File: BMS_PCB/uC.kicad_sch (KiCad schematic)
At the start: 2 parts, among them J2 Conn_01x09, U7 STM32F407G-DISC1

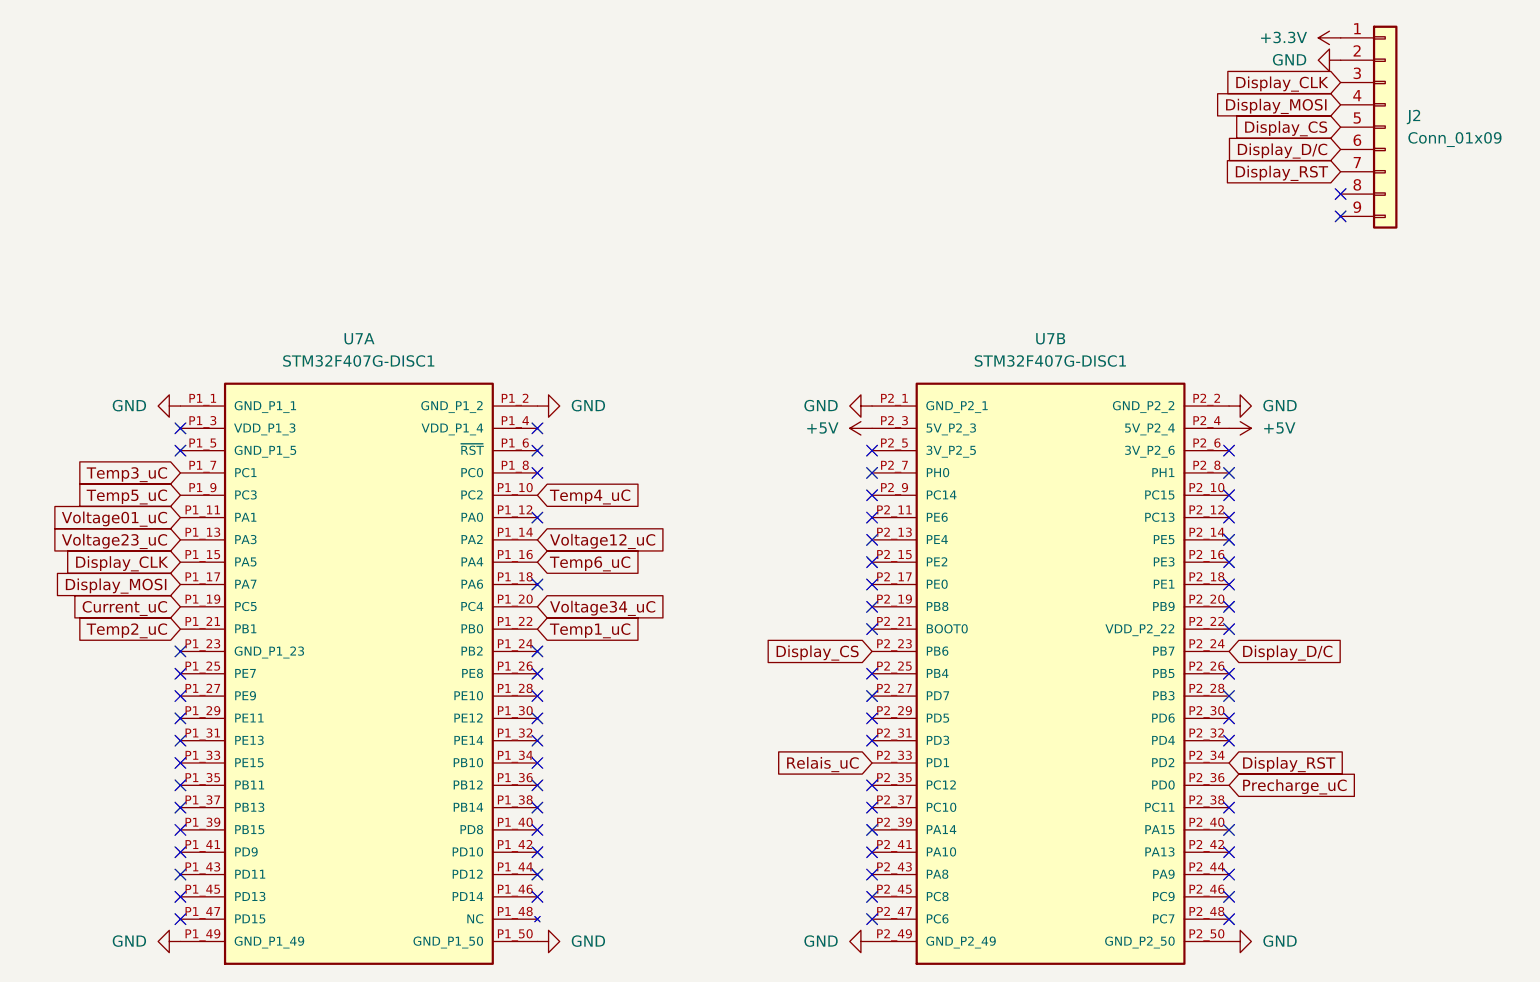
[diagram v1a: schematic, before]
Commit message: Footprints changes
-U10
-uC pins/SPI changes
- Fuses
- DSUB
- reupload layout
- etc.
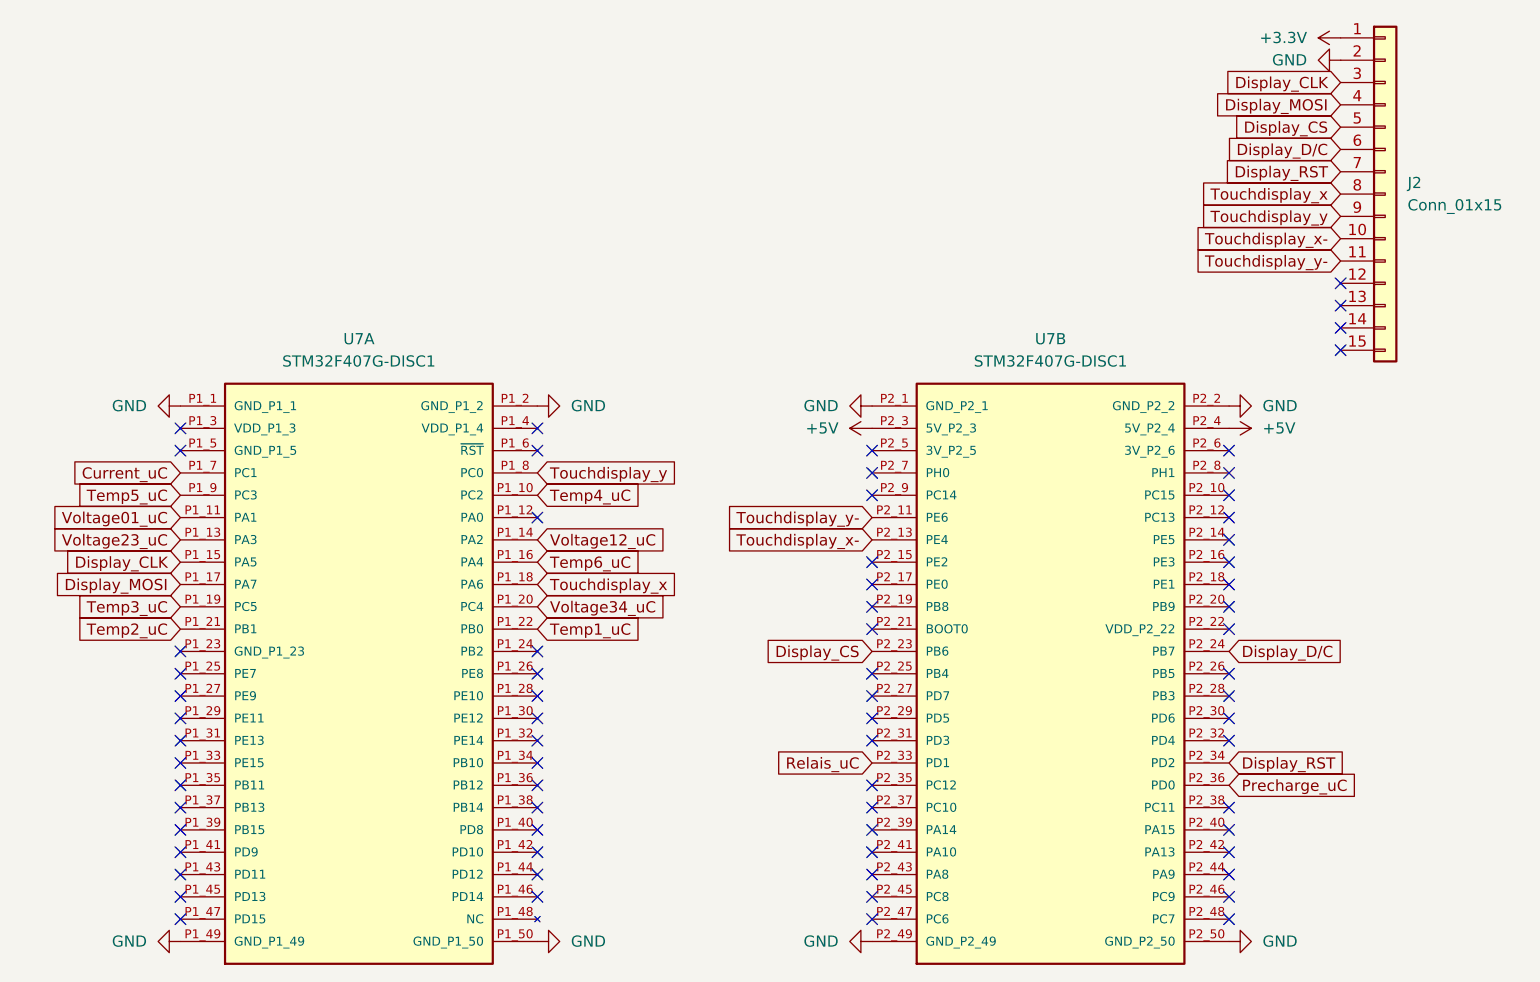
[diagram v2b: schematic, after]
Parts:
- removed J2: Conn_01x09, Connector_Dsub:DSUB-9_Socket_Horizontal_P2.77x2.84mm_EdgePinOffset14.56mm_Housed_MountingHolesOffset15.98mm, symbol Connector_Generic:Conn_01x09
- added J2: Conn_01x15, Connector_Dsub:DSUB-15_Socket_Horizontal_P2.77x2.84mm_EdgePinOffset14.56mm_Housed_MountingHolesOffset15.98mm, symbol Connector_Generic:Conn_01x15
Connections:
- net +3.3V: now also J2.1 (Pin_1)
- net Current_uC: now also U7.P1_7 (PC1); no longer U7.P1_19 (PC5)
- net Display_CLK: now also J2.3 (Pin_3)
- net Display_CS: now also J2.5 (Pin_5)
- net Display_D/C: now also J2.6 (Pin_6)
- net Display_MOSI: now also J2.4 (Pin_4)
- net Display_RST: now also J2.7 (Pin_7)
- net GND: now also J2.2 (Pin_2)
- net Temp3_uC: now also U7.P1_19 (PC5); no longer U7.P1_7 (PC1)
- net Touchdisplay_y-: now reaches U7.P2_11 (PE6)
- net Touchdisplay_y-: now also J2.11 (Pin_11)
- net Touchdisplay_x-: now reaches U7.P2_13 (PE4)
- net Touchdisplay_x-: now also J2.10 (Pin_10)
- net Touchdisplay_x: now reaches U7.P1_18 (PA6)
- net Touchdisplay_x: now also J2.8 (Pin_8)
- net Touchdisplay_y: now reaches U7.P1_8 (PC0)
- net Touchdisplay_y: now also J2.9 (Pin_9)
- no-connect marks 73 -> 71
